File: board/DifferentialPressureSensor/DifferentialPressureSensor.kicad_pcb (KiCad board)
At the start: 2 copper layers, 88.5 x 65 mm, 15 parts, among them U1 ESP32-S3-DEVKIT-LIPO

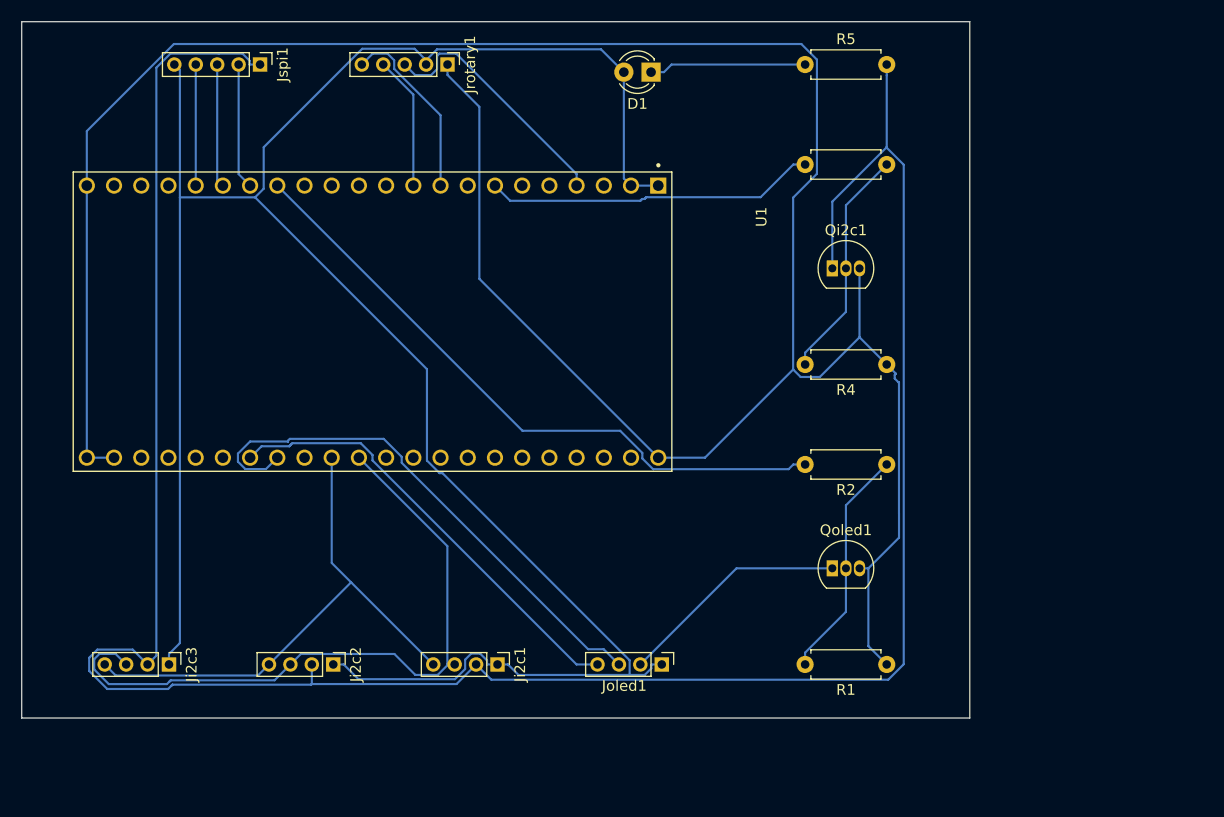
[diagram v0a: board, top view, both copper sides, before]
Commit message: doc
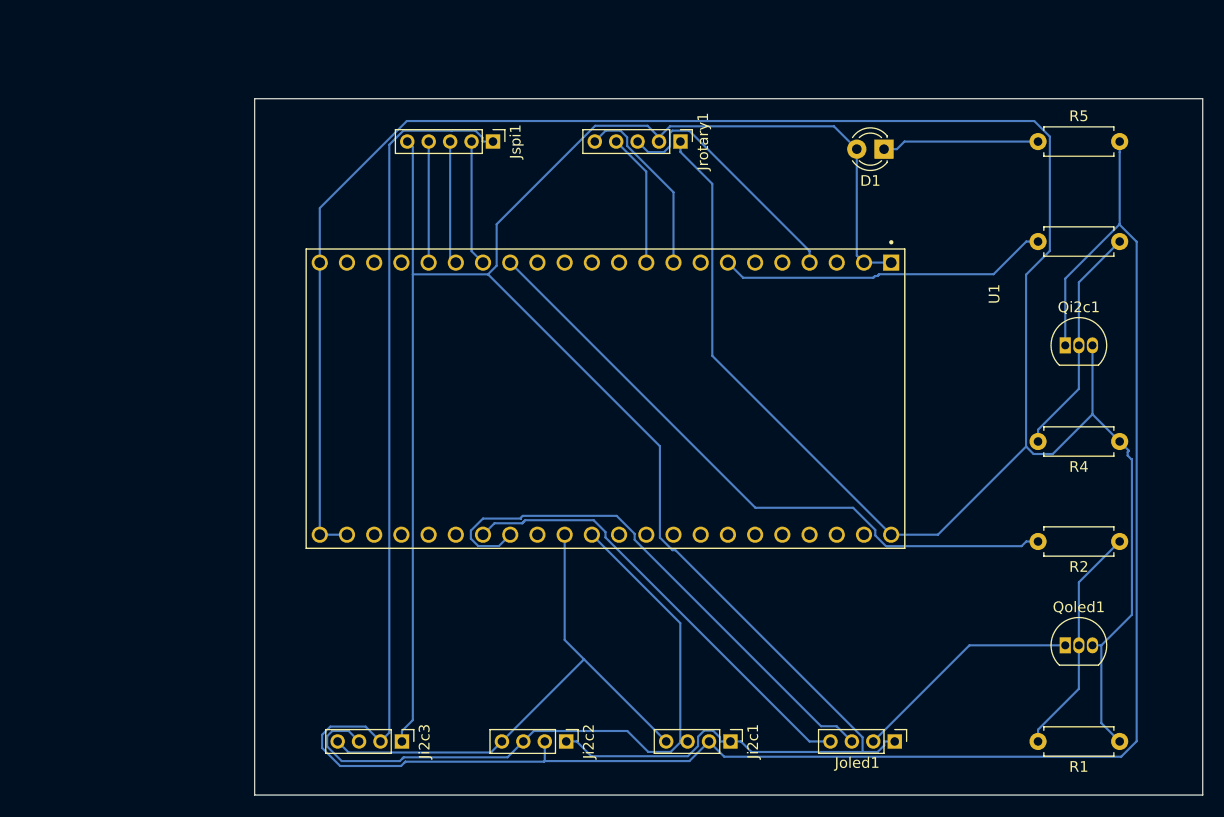
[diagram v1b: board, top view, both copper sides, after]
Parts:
- moved R5 22.9 mm to (108.1, 32.2)
- moved Ji2c1 22.9 mm to (79.4, 88.2)
- moved Ji2c2 22.9 mm to (64.1, 88.2)
- moved Ji2c3 22.9 mm to (48.7, 88.2)
- moved Jspi1 22.9 mm to (57.2, 32.2)
- moved D1 22.9 mm to (93.7, 32.9)
- moved Joled1 22.9 mm to (94.7, 88.2)
- moved Jrotary1 22.9 mm to (74.7, 32.2)
- moved Qi2c1 22.9 mm to (110.7, 51.2)
- moved Qoled1 22.9 mm to (110.7, 79.2)
- moved R1 22.9 mm to (115.7, 88.2)
- moved R2 22.9 mm to (115.7, 69.5)
- moved R3 22.9 mm to (115.7, 41.5)
- moved R4 22.9 mm to (115.7, 60.2)
- moved U1 22.9 mm to (67.7, 56.2)
